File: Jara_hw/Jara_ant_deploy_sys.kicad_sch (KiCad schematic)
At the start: 16 parts, among them J2 Conn_01x15, J3 Conn_01x10, Q1 Q_NMOS_GSD, Q2 Q_NMOS_GSD, SW3 SW_SPDT_312, SW4 SW_SPDT_312, U2 RFM95W-868S2

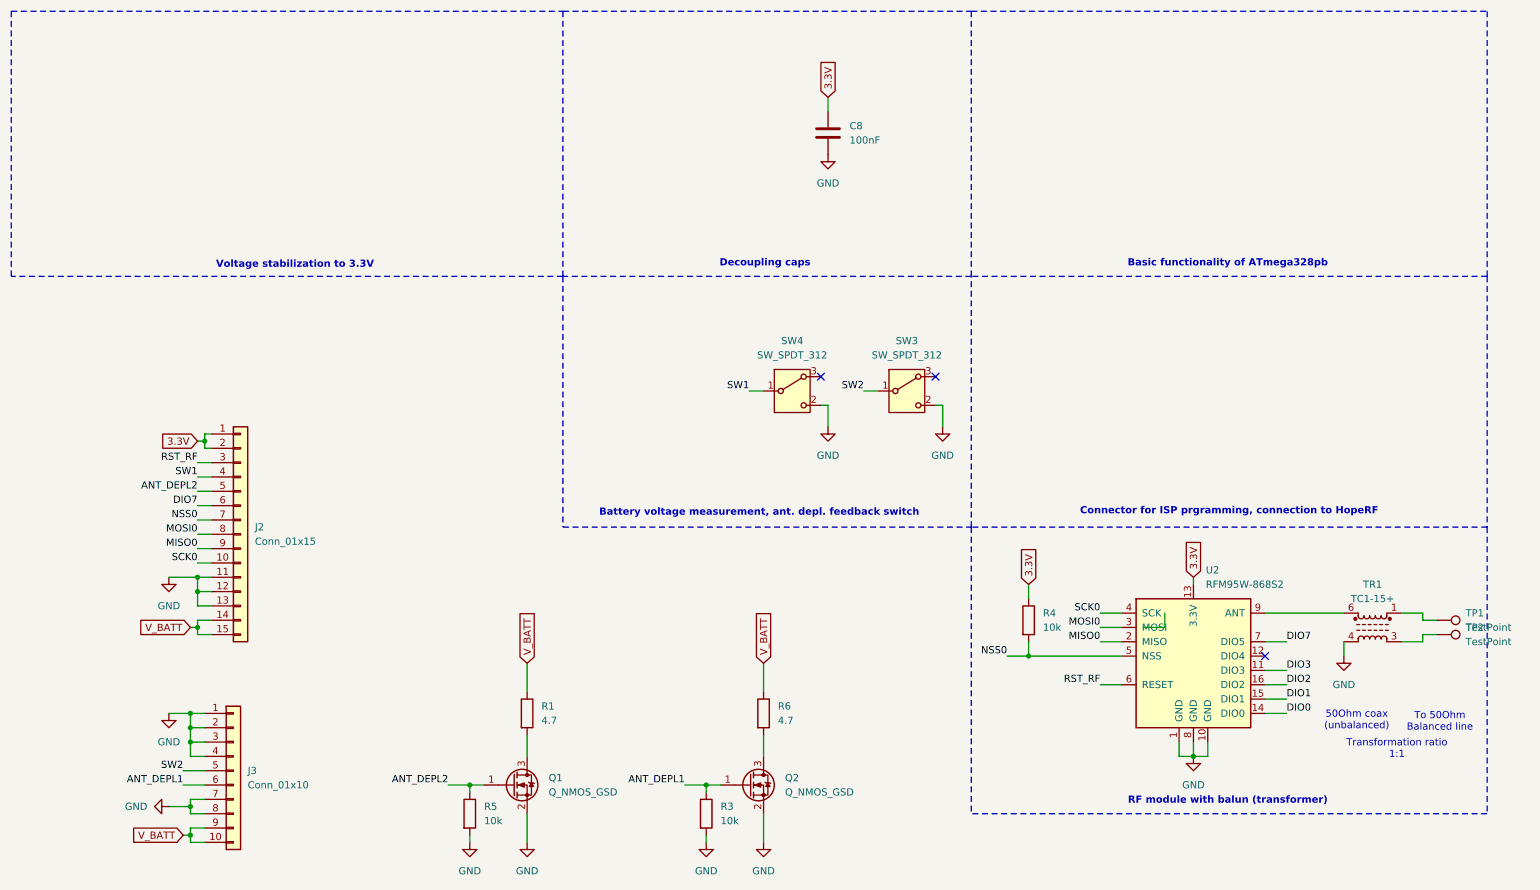
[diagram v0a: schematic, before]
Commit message: cleaning up the schematics
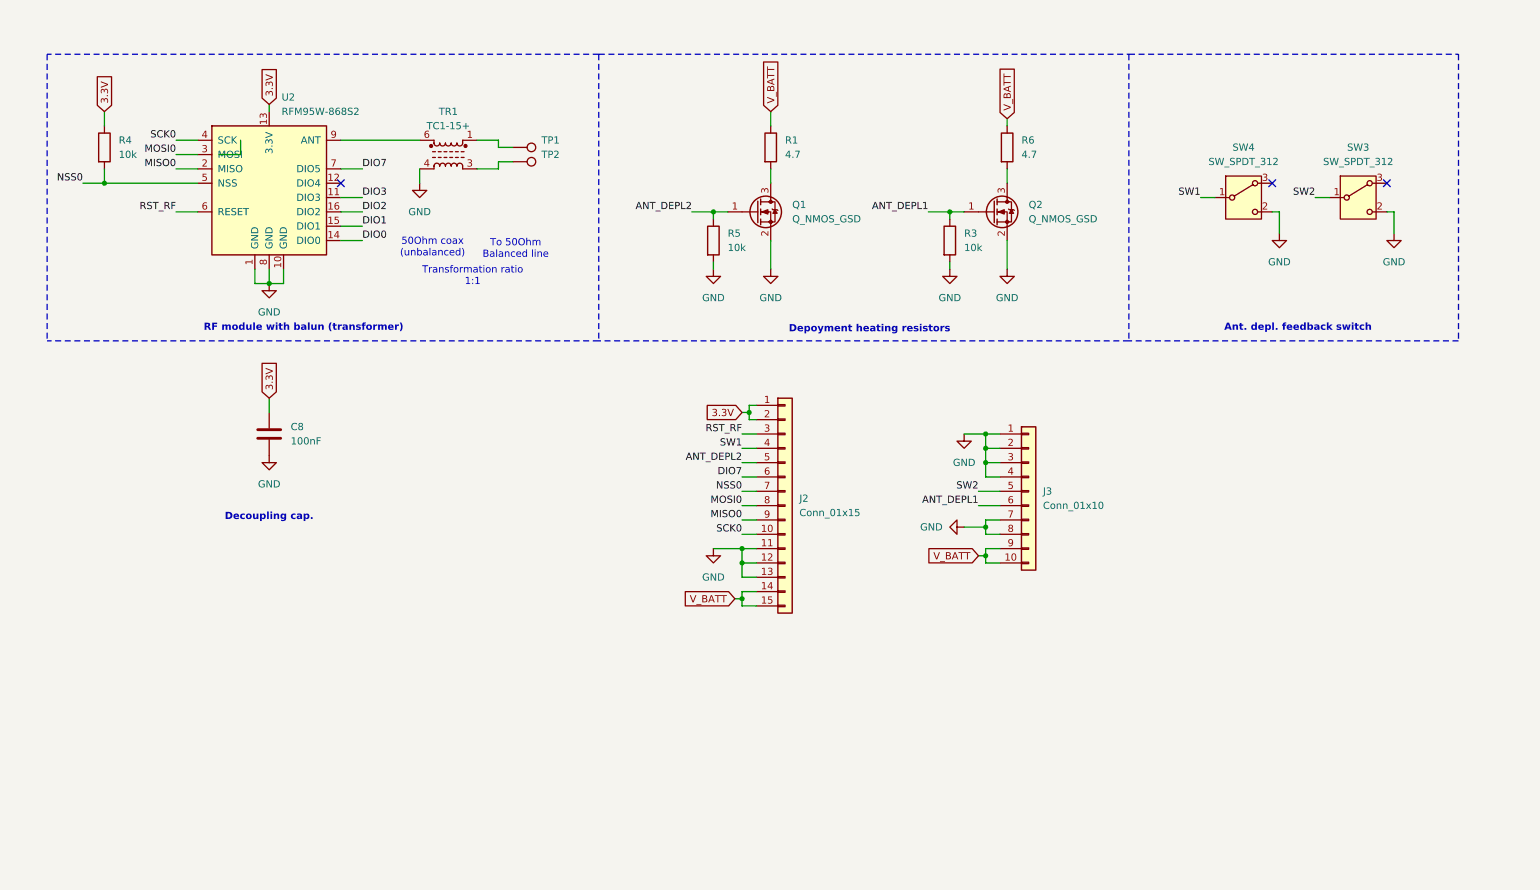
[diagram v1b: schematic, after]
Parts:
- TP1, TP2: value TestPoint -> (none)
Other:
- note added: "Ant. depl. feedback switch"
- note added: "Decoupling cap."
- note added: "Depoyment heating resistors"
- note removed: "Basic functionality of ATmega328pb"
- note removed: "Battery voltage measurement, ant. depl. feedback switch"
- note removed: "Connector for ISP prgramming, connection to HopeRF"
- note removed: "Decoupling caps"
- note removed: "Voltage stabilization to 3.3V"
- moved on the sheet: C8, J2, J3, Q1, Q2, R1, R3, R4, R5, R6, SW3, SW4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
